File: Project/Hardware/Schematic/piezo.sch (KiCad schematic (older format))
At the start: 5 parts, among them Q1 2N3906, U7 piezo

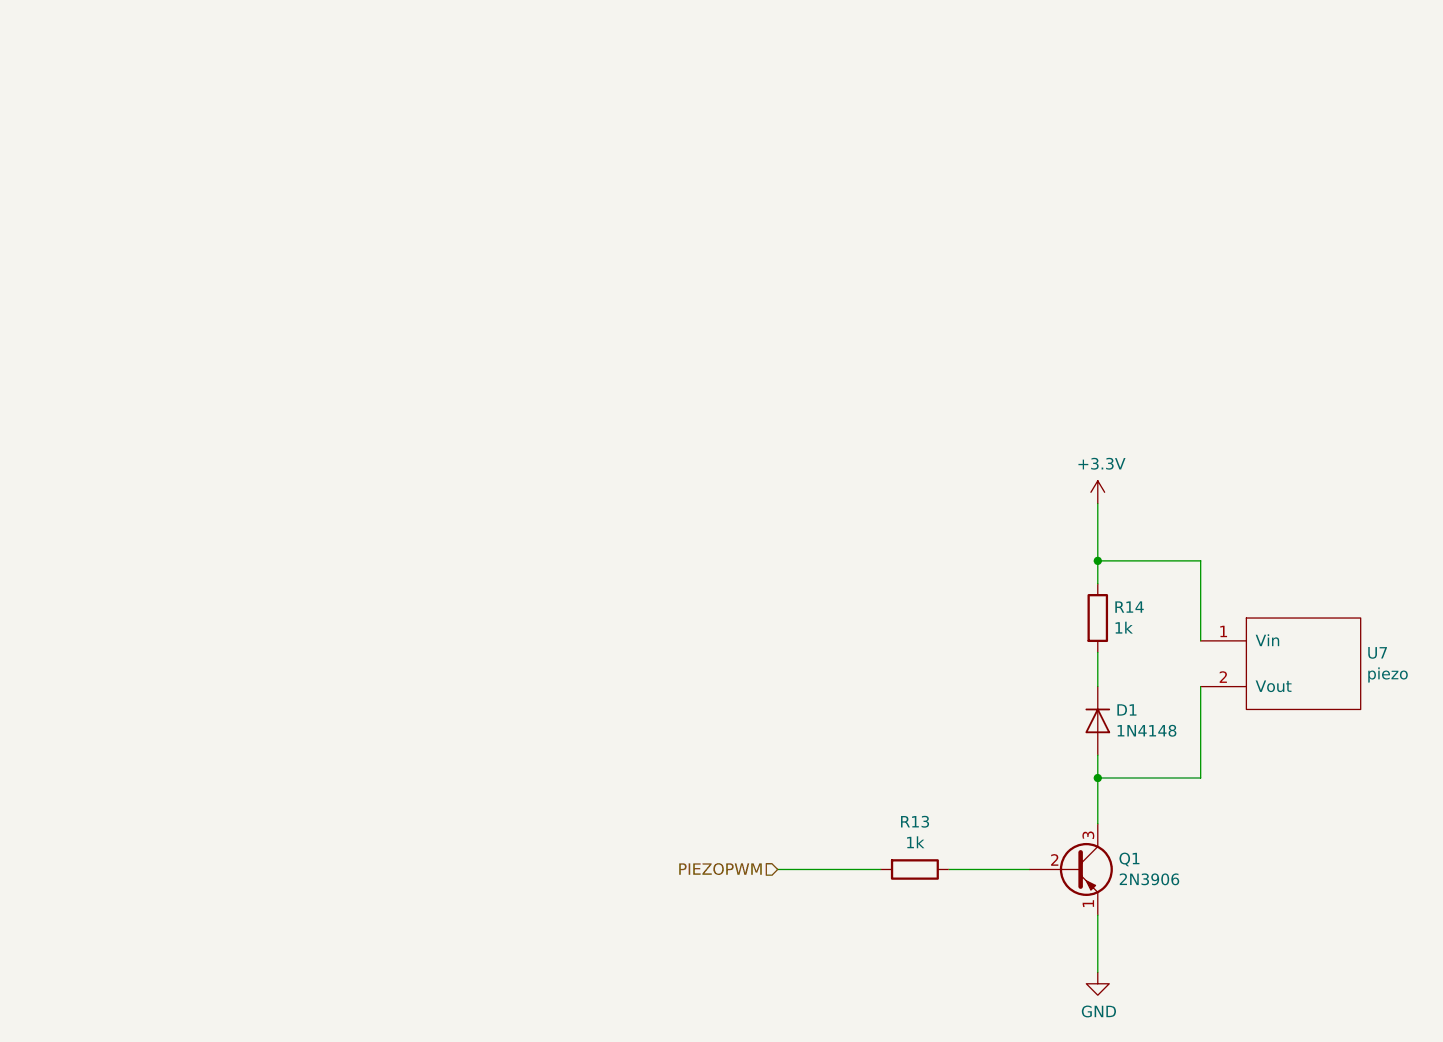
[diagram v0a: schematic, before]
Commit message: Intermediate...
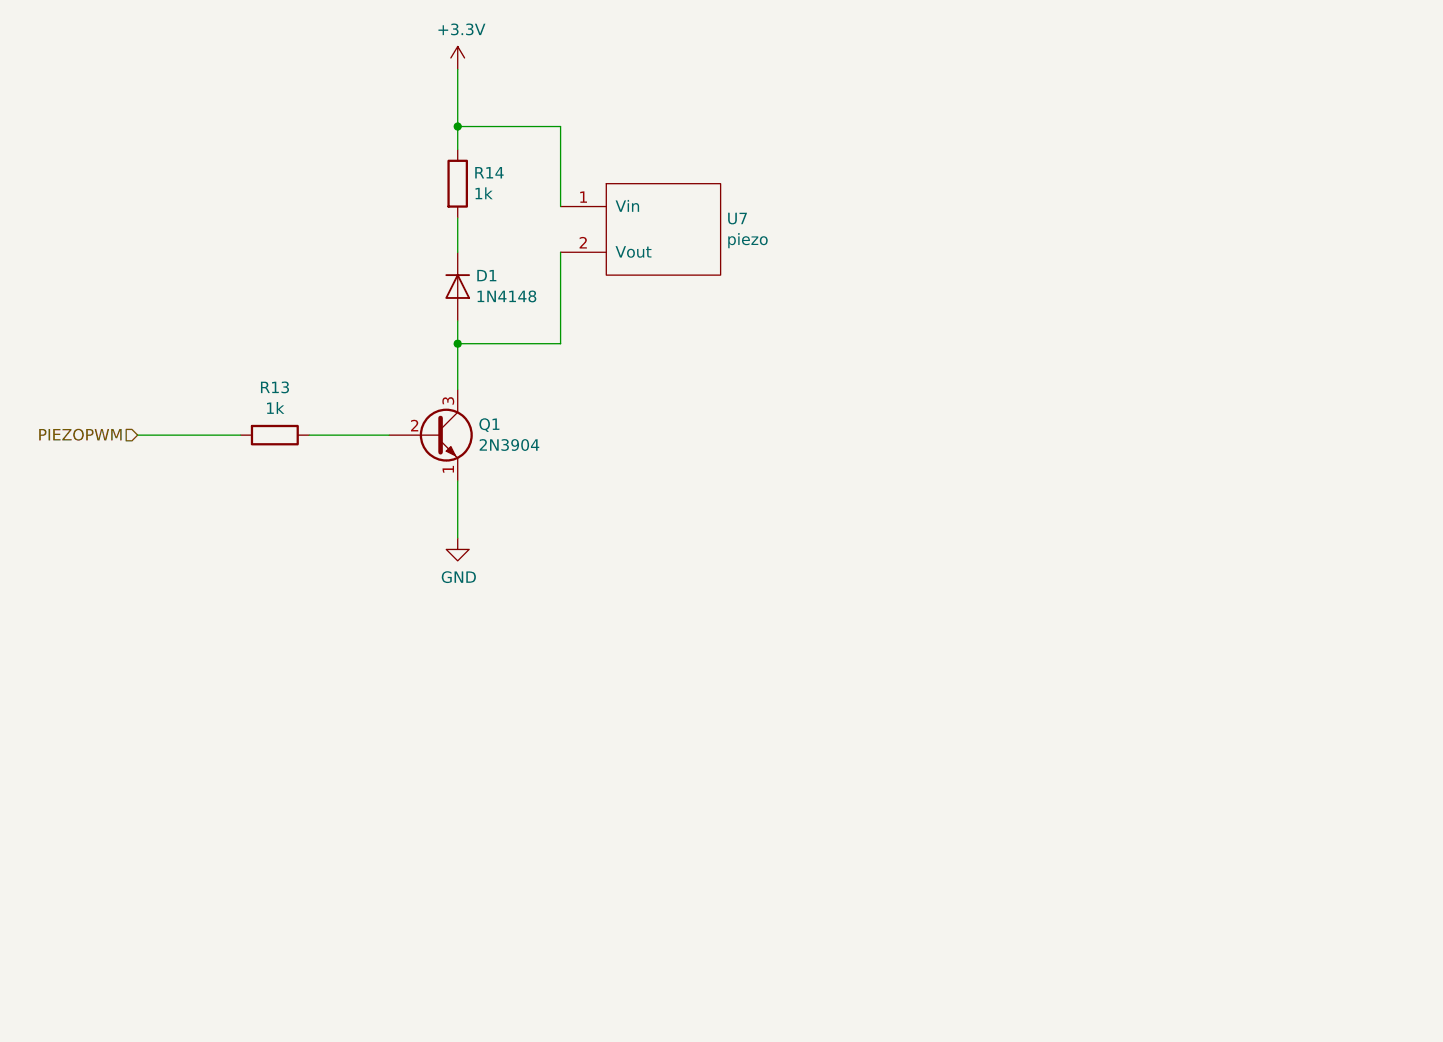
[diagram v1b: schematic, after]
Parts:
- removed Q1: 2N3906, TO_SOT_Packages_THT:TO-92_Inline_Wide, symbol Transistor_BJT:2N3906
- added Q1: 2N3904, Package_TO_SOT_THT:TO-92_Inline_Wide, symbol Transistor_BJT:2N3904
- R13, R14: footprint (none) -> Resistor_SMD:R_0805_2012Metric_Pad1.15x1.40mm_HandSolder
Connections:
- net GND: now also Q1.1 (E)
- net at D1.2 (A), U7.2 (Vout): now also Q1.3 (C)
- net at R13.1: now also Q1.2 (B)
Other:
- moved on the sheet: D1, R13, R14, U7
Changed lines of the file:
@@
 EELAYER 26 0
 EELAYER END
-$Descr A4 11693 8268
+$Descr User 5512 5512
 encoding utf-8
 Sheet 6 7
 Title ""
-Date ""
-Rev ""
-Comp ""
+Date "2019-02-12"
+Rev "1"
+Comp "PASC"
 Comment1 ""
 Comment2 ""
@@
 L PASC:piezo U7
 U 1 1 5C5E3EC0
-P 6600 3700
-F 0 "U7" H 6877 3746 50  0000 L CNN
-F 1 "piezo" H 6877 3655 50  0000 L CNN
-F 2 "PASC:Piezo" H 6600 3700 50  0001 C CNN
-F 3 "" H 6600 3700 50  0001 C CNN
-	1    6600 3700
+P 3800 1800
+F 0 "U7" H 4077 1846 50  0000 L CNN
+F 1 "piezo" H 4077 1755 50  0000 L CNN
+F 2 "PASC:Piezo" H 3800 1800 50  0001 C CNN
+F 3 "" H 3800 1800 50  0001 C CNN
+	1    3800 1800
 	1    0    0    -1
 $EndComp
@@
 L Device:R R14
 U 1 1 5C5EB38A
-P 5700 3500
-F 0 "R14" H 5770 3546 50  0000 L CNN
-F 1 "1k" H 5770 3455 50  0000 L CNN
-F 2 "" V 5630 3500 50  0001 C CNN
-F 3 "~" H 5700 3500 50  0001 C CNN
-	1    5700 3500
+P 2900 1600
+F 0 "R14" H 2970 1646 50  0000 L CNN
+F 1 "1k" H 2970 1555 50  0000 L CNN
+F 2 "Resistor_SMD:R_0805_2012Metric_Pad1.15x1.40mm_HandSolder" V 2830 1600 50  0001 C CNN
+F 3 "~" H 2900 1600 50  0001 C CNN
+	1    2900 1600
 	1    0    0    -1
 $EndComp
@@
 L Diode:1N4148 D1
 U 1 1 5C5EB4E1
-P 5700 3950
-F 0 "D1" V 5654 4029 50  0000 L CNN
-F 1 "1N4148" V 5745 4029 50  0000 L CNN
-F 2 "Diode_THT:D_DO-35_SOD27_P7.62mm_Horizontal" H 5700 3775 50  0001 C CNN
-F 3 "http://www.nxp.com/documents/data_sheet/1N4148_1N4448.pdf" H 5700 3950 50  0001 C CNN
-	1    5700 3950
+P 2900 2050
+F 0 "D1" V 2854 2129 50  0000 L CNN
+F 1 "1N4148" V 2945 2129 50  0000 L CNN
+F 2 "Diode_THT:D_DO-35_SOD27_P7.62mm_Horizontal" H 2900 1875 50  0001 C CNN
+F 3 "http://www.nxp.com/documents/data_sheet/1N4148_1N4448.pdf" H 2900 2050 50  0001 C CNN
+	1    2900 2050
 	0    1    1    0
 $EndComp
 Wire Wire Line
-	5700 3000 5700 3250
+	2900 1100 2900 1350
 Wire Wire Line
-	5700 3650 5700 3800
+	2900 1750 2900 1900
 Wire Wire Line
-	5700 4100 5700 4200
+	2900 2200 2900 2300
 Wire Wire Line
-	6150 3600 6150 3250
+	3350 1700 3350 1350
 Wire Wire Line
-	6150 3250 5700 3250
-Connection ~ 5700 3250
+	3350 1350 2900 1350
+Connection ~ 2900 1350
 Wire Wire Line
-	5700 3250 5700 3350
+	2900 1350 2900 1450
 Wire Wire Line
-	6150 3800 6150 4200
+	3350 1900 3350 2300
 Wire Wire Line
-	6150 4200 5700 4200
-Connection ~ 5700 4200
+	3350 2300 2900 2300
+Connection ~ 2900 2300
 Wire Wire Line
-	5700 4200 5700 4400
+	2900 2300 2900 2500
 $Comp
 L Device:R R13
 U 1 1 5C5EB823
-P 4900 4600
-F 0 "R13" V 4693 4600 50  0000 C CNN
-F 1 "1k" V 4784 4600 50  0000 C CNN
-F 2 "" V 4830 4600 50  0001 C CNN
-F 3 "~" H 4900 4600 50  0001 C CNN
-	1    4900 4600
+P 2100 2700
+F 0 "R13" V 1893 2700 50  0000 C CNN
+F 1 "1k" V 1984 2700 50  0000 C CNN
+F 2 "Resistor_SMD:R_0805_2012Metric_Pad1.15x1.40mm_HandSolder" V 2030 2700 50  0001 C CNN
+F 3 "~" H 2100 2700 50  0001 C CNN
+	1    2100 2700
 	0    1    1    0
 $EndComp
 Wire Wire Line
-	5050 4600 5400 4600
+	2250 2700 2600 2700
 $Comp
 L power:GND #PWR0137
 U 1 1 5C5EB928
-P 5700 5050
-F 0 "#PWR0137" H 5700 4800 50  0001 C CNN
-F 1 "GND" H 5705 4877 50  0000 C CNN
-F 2 "" H 5700 5050 50  0001 C CNN
-F 3 "" H 5700 5050 50  0001 C CNN
-	1    5700 5050
+P 2900 3150
+F 0 "#PWR0137" H 2900 2900 50  0001 C CNN
+F 1 "GND" H 2905 2977 50  0000 C CNN
+F 2 "" H 2900 3150 50  0001 C CNN
+F 3 "" H 2900 3150 50  0001 C CNN
+	1    2900 3150
 	1    0    0    -1
 $EndComp
 Wire Wire Line
-	5700 4800 5700 5050
+	2900 2900 2900 3150
 Wire Wire Line
-	4750 4600 4300 4600
-Text HLabel 4300 4600 0    50   Input ~ 0
+	1950 2700 1500 2700
+Text HLabel 1500 2700 0    50   Input ~ 0
 PIEZOPWM
 $Comp
-L Transistor_BJT:2N3906 Q1
-U 1 1 5C68E108
-P 5600 4600
-F 0 "Q1" H 5791 4646 50  0000 L CNN
-F 1 "2N3906" H 5791 4555 50  0000 L CNN
-F 2 "TO_SOT_Packages_THT:TO-92_Inline_Wide" H 5800 4525 50  0001 L CIN
-F 3 "https://www.fairchildsemi.com/datasheets/2N/2N3906.pdf" H 5600 4600 50  0001 L CNN
-	1    5600 4600
+L power:+3.3V #PWR0138
+U 1 1 5C6DC10D
+P 2900 1100
+F 0 "#PWR0138" H 2900 950 50  0001 C CNN
+F 1 "+3.3V" H 2915 1273 50  0000 C CNN
+F 2 "" H 2900 1100 50  0001 C CNN
+F 3 "" H 2900 1100 50  0001 C CNN
+	1    2900 1100
 	1    0    0    -1
 $EndComp
 $Comp
-L power:+3.3V #PWR0138
-U 1 1 5C6DC10D
-P 5700 3000
-F 0 "#PWR0138" H 5700 2850 50  0001 C CNN
-F 1 "+3.3V" H 5715 3173 50  0000 C CNN
-F 2 "" H 5700 3000 50  0001 C CNN
-F 3 "" H 5700 3000 50  0001 C CNN
-	1    5700 3000
+L Transistor_BJT:2N3904 Q1
+U 1 1 5C64EC5C
+P 2800 2700
+F 0 "Q1" H 2991 2746 50  0000 L CNN
+F 1 "2N3904" H 2991 2655 50  0000 L CNN
+F 2 "Package_TO_SOT_THT:TO-92_Inline_Wide" H 3000 2625 50  0001 L CIN
+F 3 "https://www.fairchildsemi.com/datasheets/2N/2N3904.pdf" H 2800 2700 50  0001 L CNN
+	1    2800 2700
 	1    0    0    -1
 $EndComp
